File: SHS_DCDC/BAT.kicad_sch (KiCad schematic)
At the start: 11 parts, among them Q10 PMV100XPEAR, Q11 PMV100XPEAR, Q12 PMV100XPEAR, Q17 PMV100XPEAR, Q9 PMV100XPEAR, U2 INA181, U7 MCP101

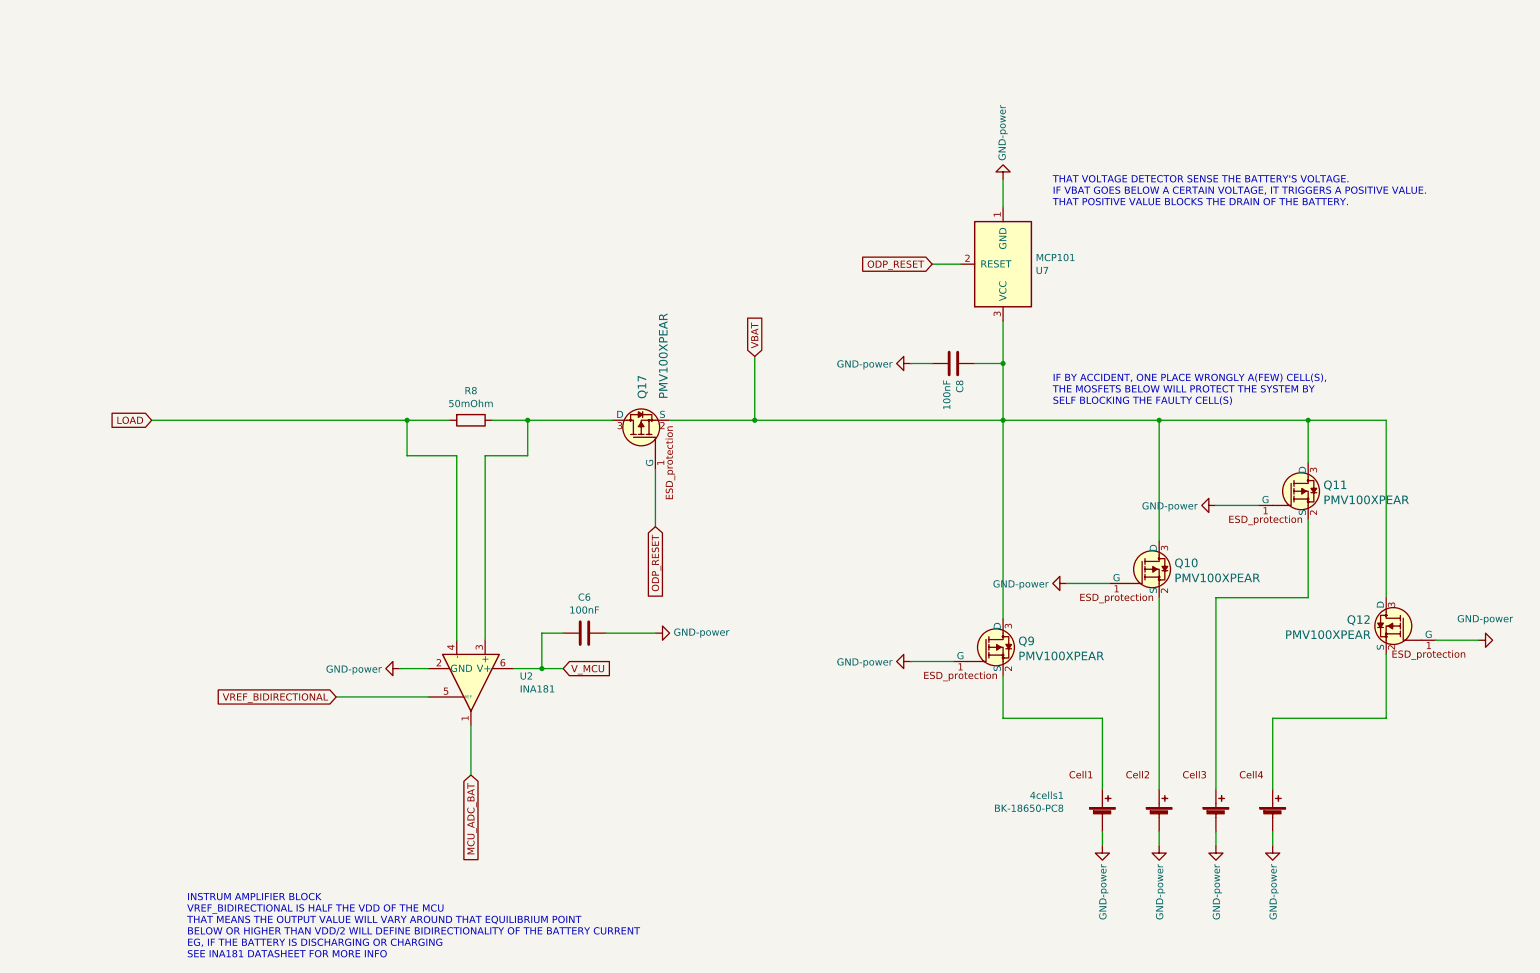
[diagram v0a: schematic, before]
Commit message: ProgressMisc
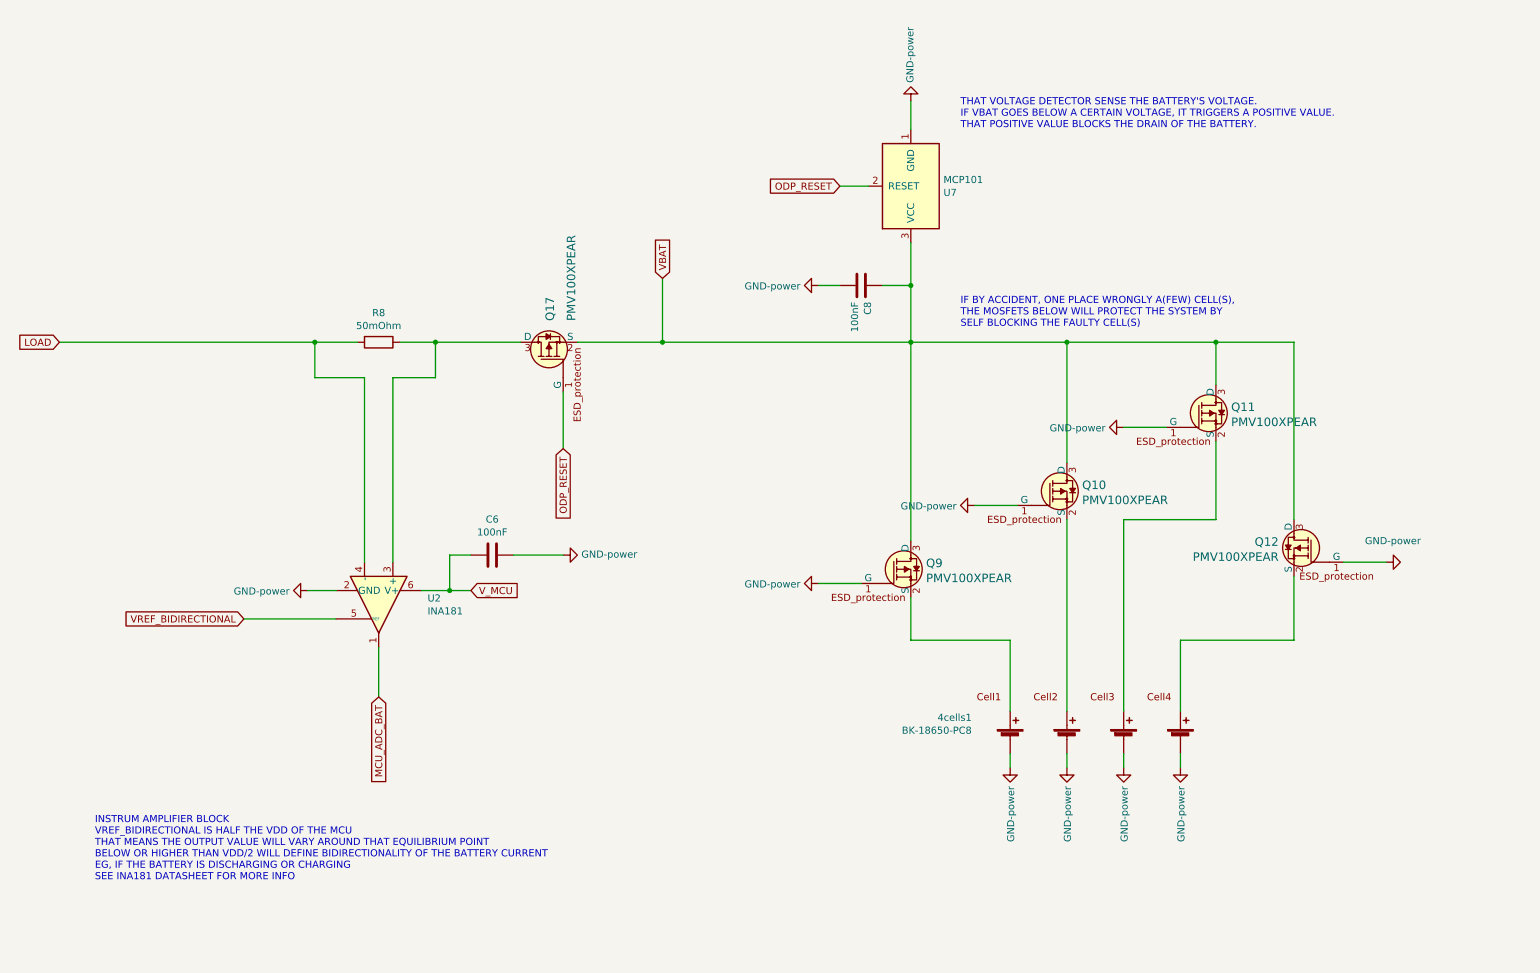
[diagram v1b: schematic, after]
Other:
- moved on the sheet: 4cells1, C6, C8, Q10, Q11, Q12, Q17, Q9, R8, U2, U7
